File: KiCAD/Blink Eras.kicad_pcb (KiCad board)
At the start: 2 copper layers, 27.9 x 20.3 mm, 12 parts, among them P1 ISP, U1 ICM7555, U2 ATTINY85-M

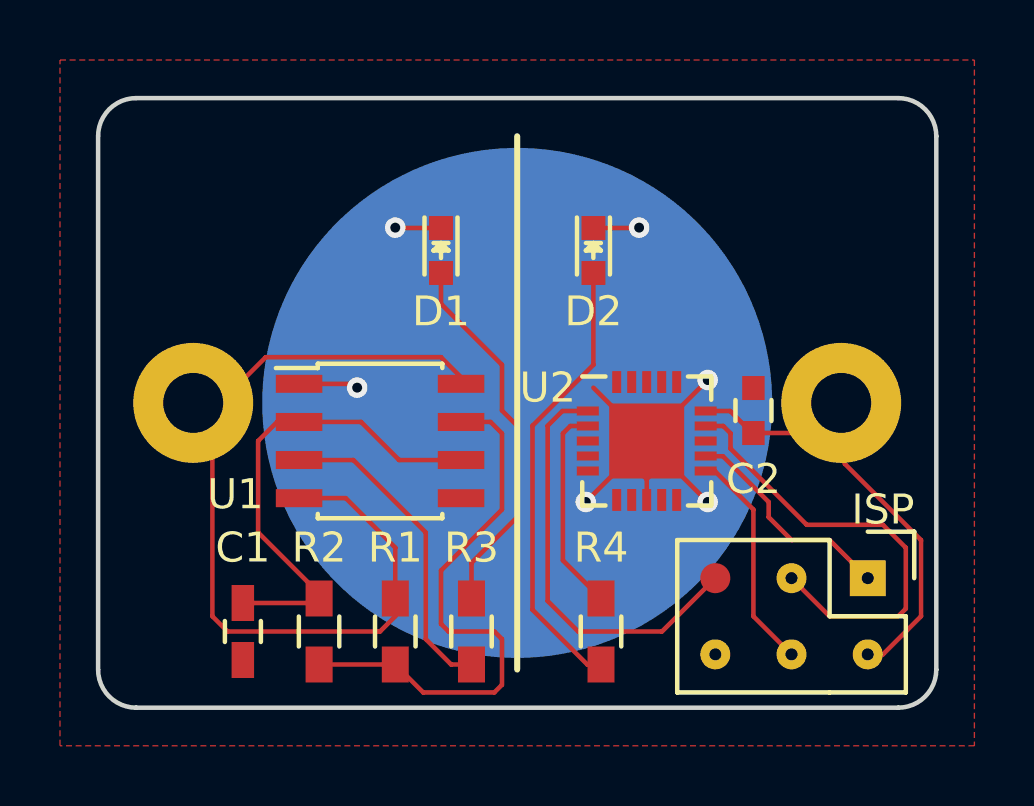
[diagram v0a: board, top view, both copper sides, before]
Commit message: Artwork, first draft..
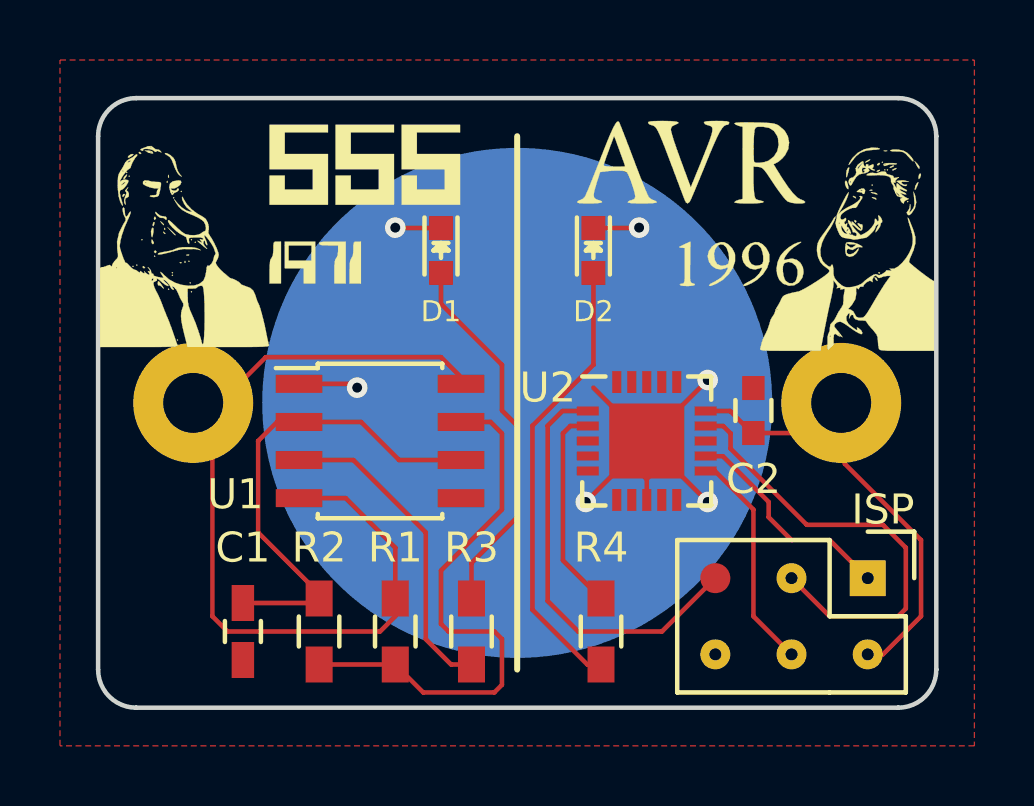
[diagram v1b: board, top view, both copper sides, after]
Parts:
- added G***: LOGO, BlinkyFeet:555-lettering, F.Cu at (137.2, 94.0)
- added G***: LOGO, BlinkyFeet:AVR-lettering, F.Cu at (152.4, 94.0)
- added G***: LOGO, BlinkyFeet:Nixon-image, F.Cu at (135.9, 95.2)
- added G***: LOGO, BlinkyFeet:Clinton-image, F.Cu at (153.7, 95.2)
